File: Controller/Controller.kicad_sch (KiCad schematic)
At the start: 40 parts, among them SW2 SW_Push, SW3 SW_Push, SW4 SW_Push, SW5 SW_Push, SW6 SW_Push, SW7 SW_Push, SW8 SW_Push, SW9 SW_Push

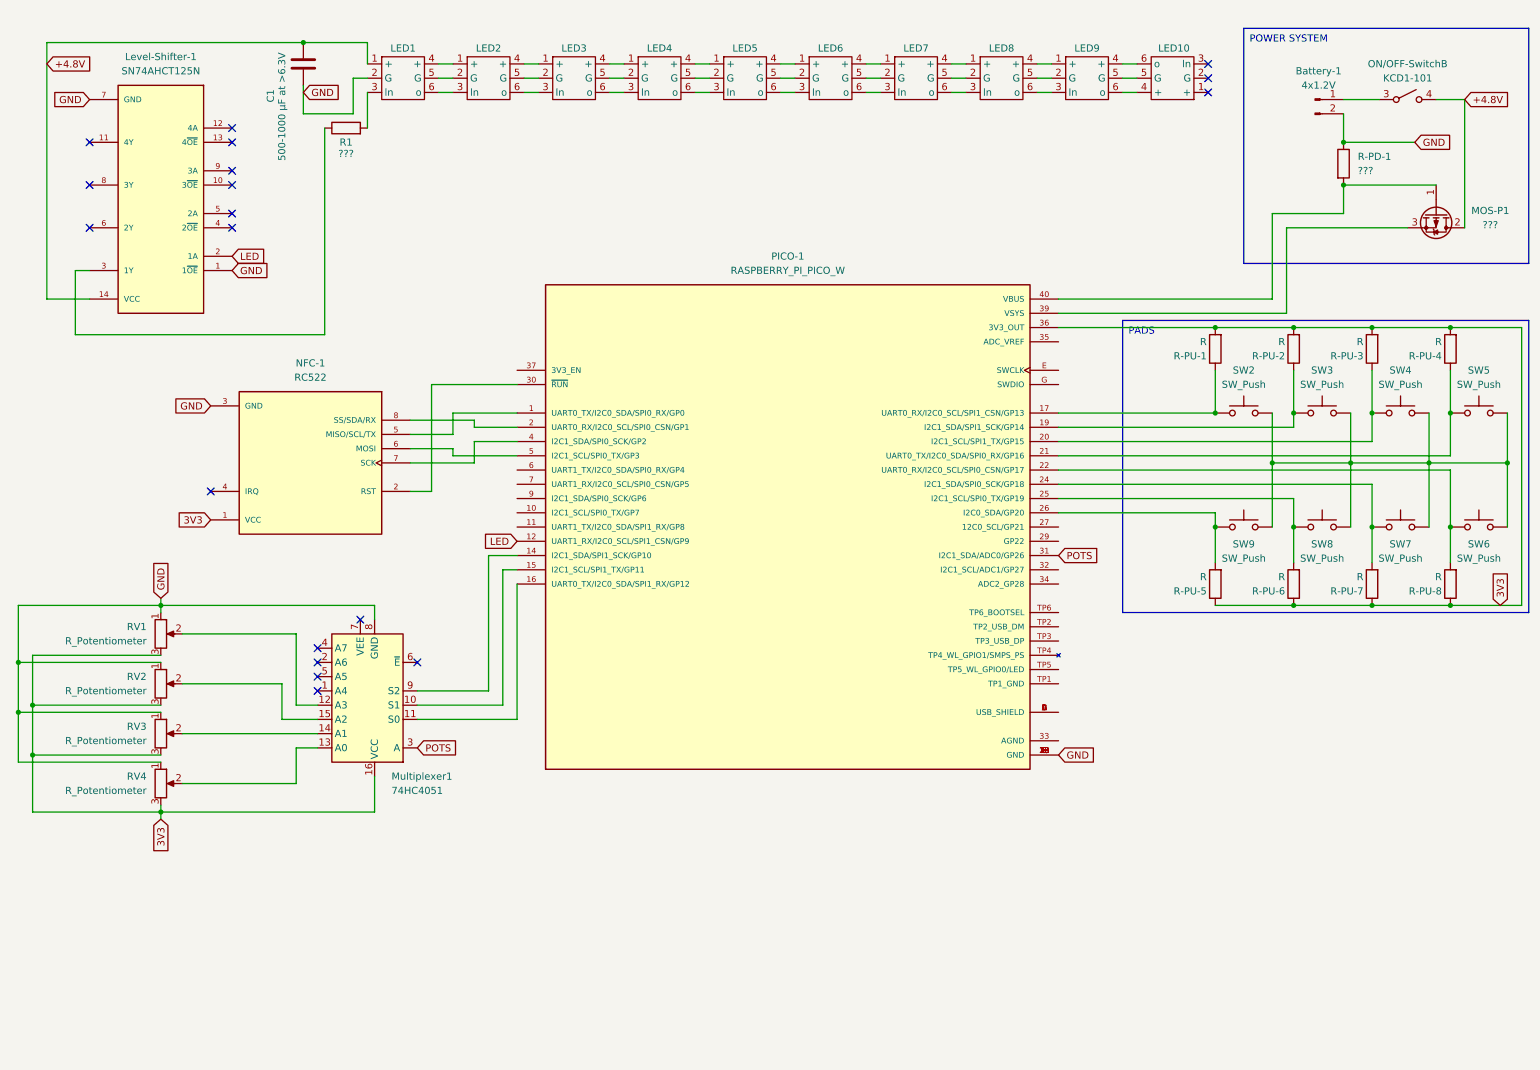
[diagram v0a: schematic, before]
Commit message: Add sections
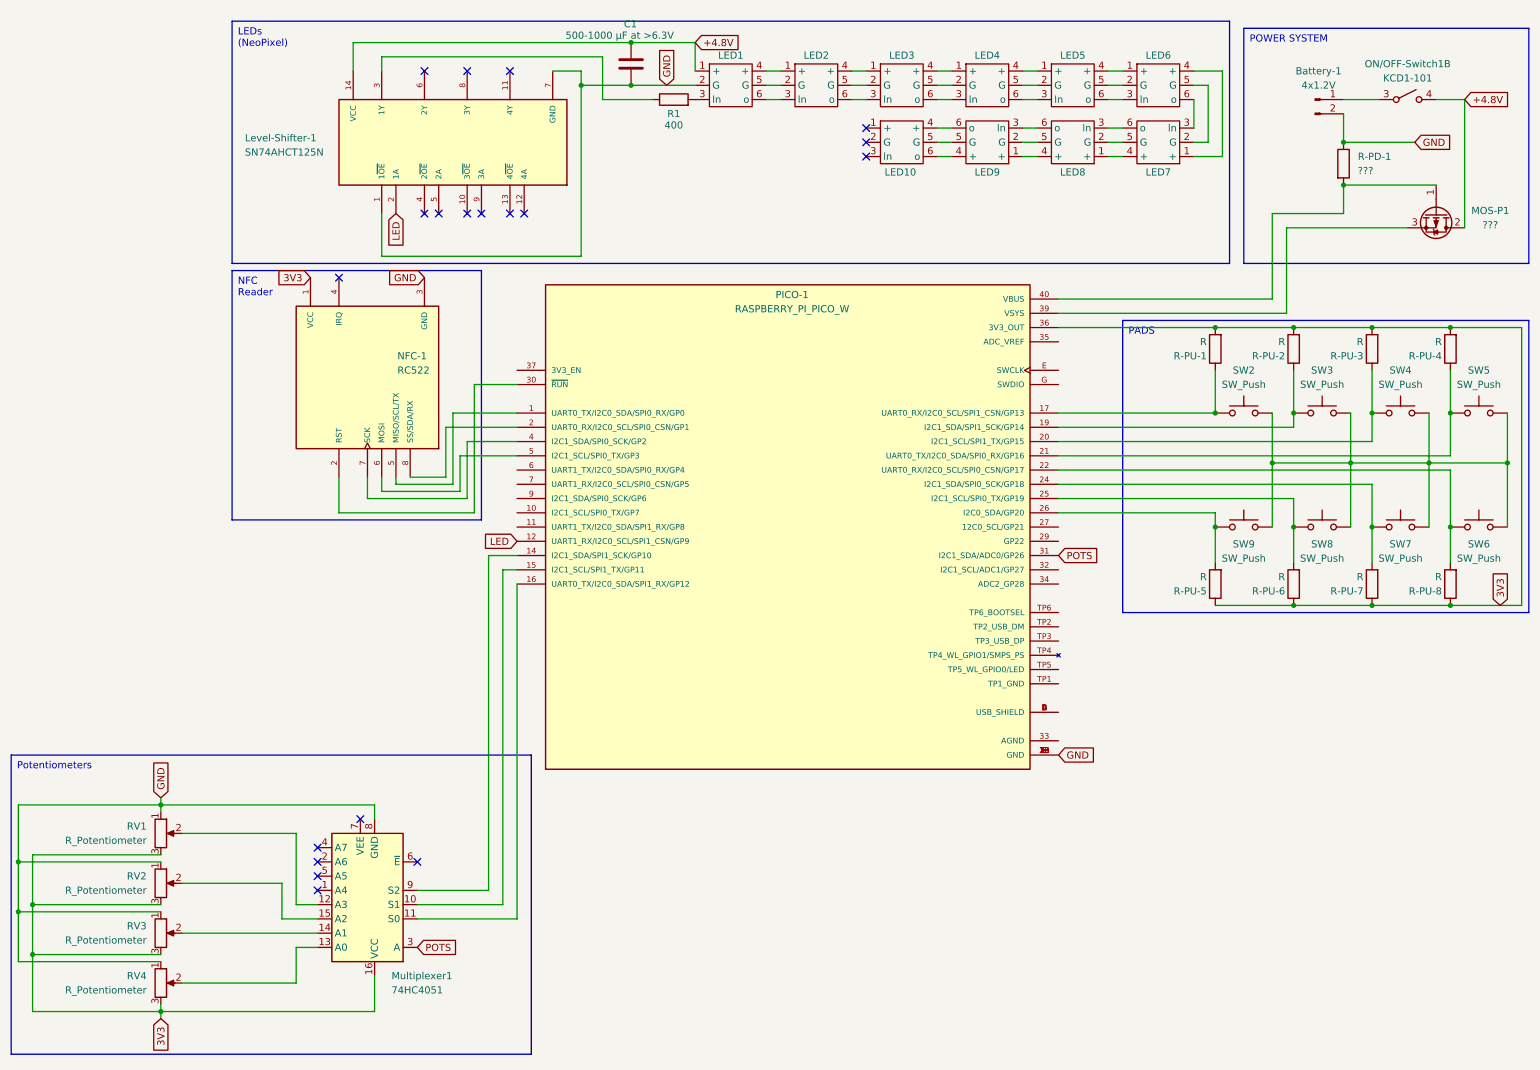
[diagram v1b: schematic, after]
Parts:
- R1: value ??? -> 400
- renumbered ON/OFF-Switch to ON/OFF-Switch1
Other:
- moved on the sheet: C1, LED1, LED10, LED2, LED3, LED4, LED5, LED6, LED7, LED8, LED9, Level-Shifter-1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
